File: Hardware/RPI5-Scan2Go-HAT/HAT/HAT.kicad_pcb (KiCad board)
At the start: 2 copper layers, 76 x 96.5 mm, 35 parts, among them J1 RPi_GPIO, J10 Conn_01x02_Socket, J12 Conn_01x02_Socket, J13 Conn_01x02_Socket, J14 Conn_01x02_Socket, J15 Jack-DC 5V, J18 Conn_01x02_Socket, J19 Conn_01x02_Socket, J2 Conn_01x04_Socket, J20 Conn_01x05_Socket, J21 Conn_01x05_Socket, J22 Conn_01x02_Socket, J23 Conn_01x04_Socket, J24 Conn_01x02_Socket, J3 Conn_01x14_Socket, J4 Conn_01x03_Socket, J5 Conn_01x03_Socket, J6 Conn_01x03_Socket, J7 Conn_01x04_Socket, J8 Conn_01x02_Socket, J9 Conn_01x02_Socket, Q1 DMG2305UX, U1 Pico

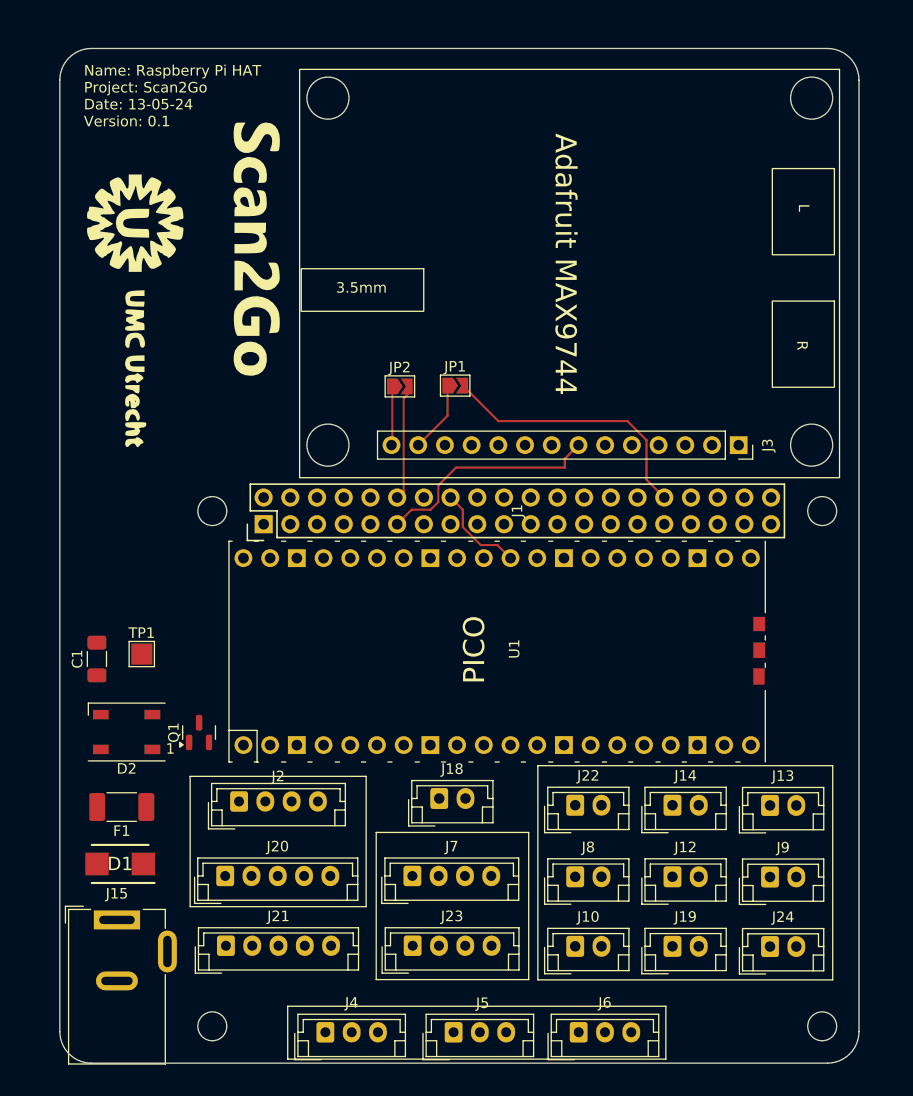
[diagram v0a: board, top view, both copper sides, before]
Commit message: V0.1 of pcb finished (To be reviewed)
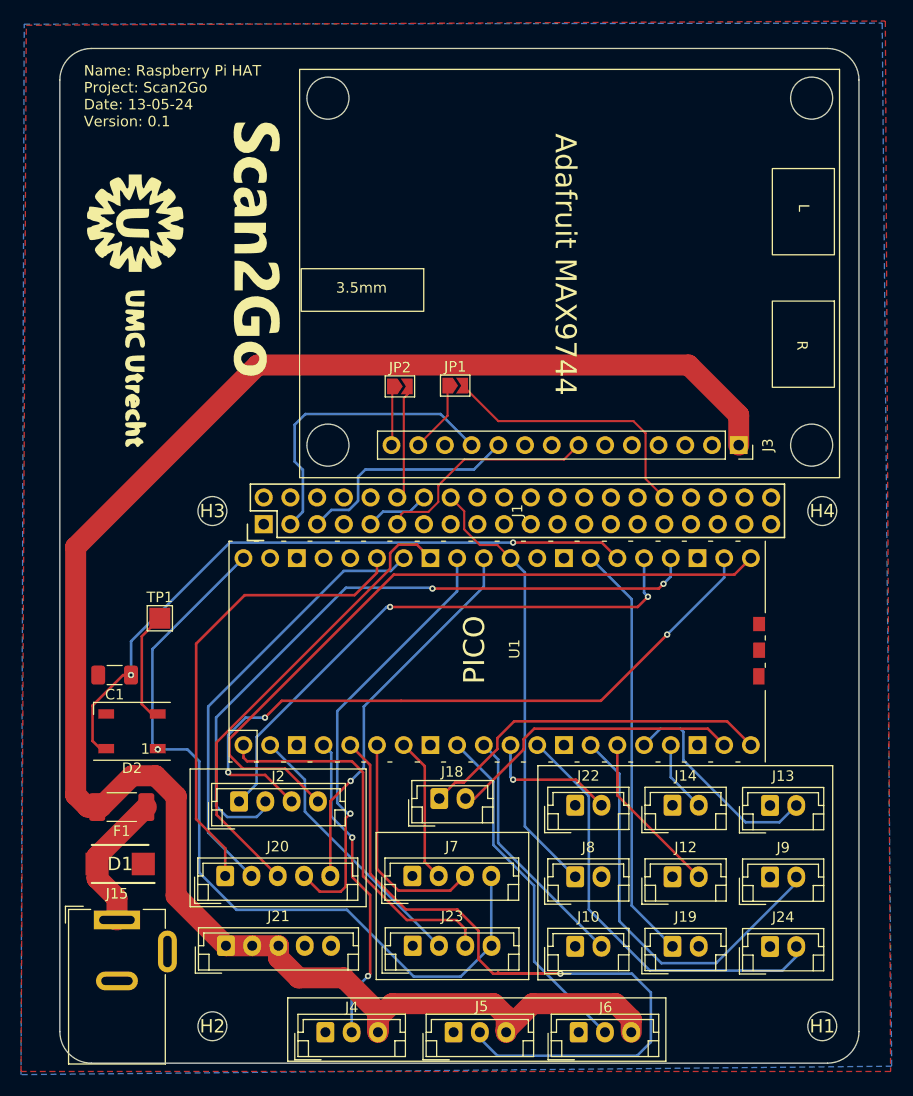
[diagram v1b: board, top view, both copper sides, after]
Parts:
- removed ? (x4): , RPi_Hat:RPi_Hat_Mounting_Hole
- removed Q1: DMG2305UX, Package_TO_SOT_SMD:SOT-23
- added H1: MountingHole, , F.Cu at (179.6, 144.9)
- added H2: MountingHole, , F.Cu at (121.6, 144.9)
- added H3: MountingHole, , F.Cu at (121.6, 95.9)
- added H4: MountingHole, , F.Cu at (179.6, 95.9)
- moved TP1 3.81 mm to (116.6, 106.1)
- moved C1 2.27 mm to (112.3, 111.5), turned to 180 degrees
- moved D2 0.50 mm to (114.0, 116.8)
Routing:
- net +5V: track 0.00 -> 177.7 mm
- net /VBUS: track 0.00 -> 76.8 mm, vias 0 -> 1
- net Net-(J5-Pin_2): track 0.00 -> 74.9 mm, vias 0 -> 1
- net Net-(J2-Pin_4): track 0.00 -> 68.5 mm
- net Net-(J2-Pin_3): track 0.00 -> 66.0 mm, vias 0 -> 3
- net Net-(J2-Pin_2): track 0.00 -> 65.1 mm, vias 0 -> 2
- net Net-(D2-DIN): track 0.00 -> 63.3 mm, vias 0 -> 2
- net Net-(J2-Pin_1): track 0.00 -> 53.4 mm, vias 0 -> 2
- net Net-(J20-Pin_3): track 0.00 -> 44.6 mm
- net Net-(J20-Pin_1): track 0.00 -> 44.6 mm
- net Net-(J20-Pin_2): track 0.00 -> 42.3 mm
- net Net-(J20-Pin_4): track 0.00 -> 41.6 mm, vias 0 -> 1
- net Net-(J24-Pin_2): track 0.00 -> 41.3 mm
- net Net-(J19-Pin_1): track 0.00 -> 40.1 mm
- net Net-(J9-Pin_2): track 0.00 -> 40.1 mm
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- added copper zone on B.Cu, net GND
- added copper zone on F.Cu, net GND
